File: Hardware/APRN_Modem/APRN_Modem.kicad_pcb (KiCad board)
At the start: 2 copper layers, 12 parts, among them J201 Conn_Coaxial, U201 VS1003, U202 DRA818V

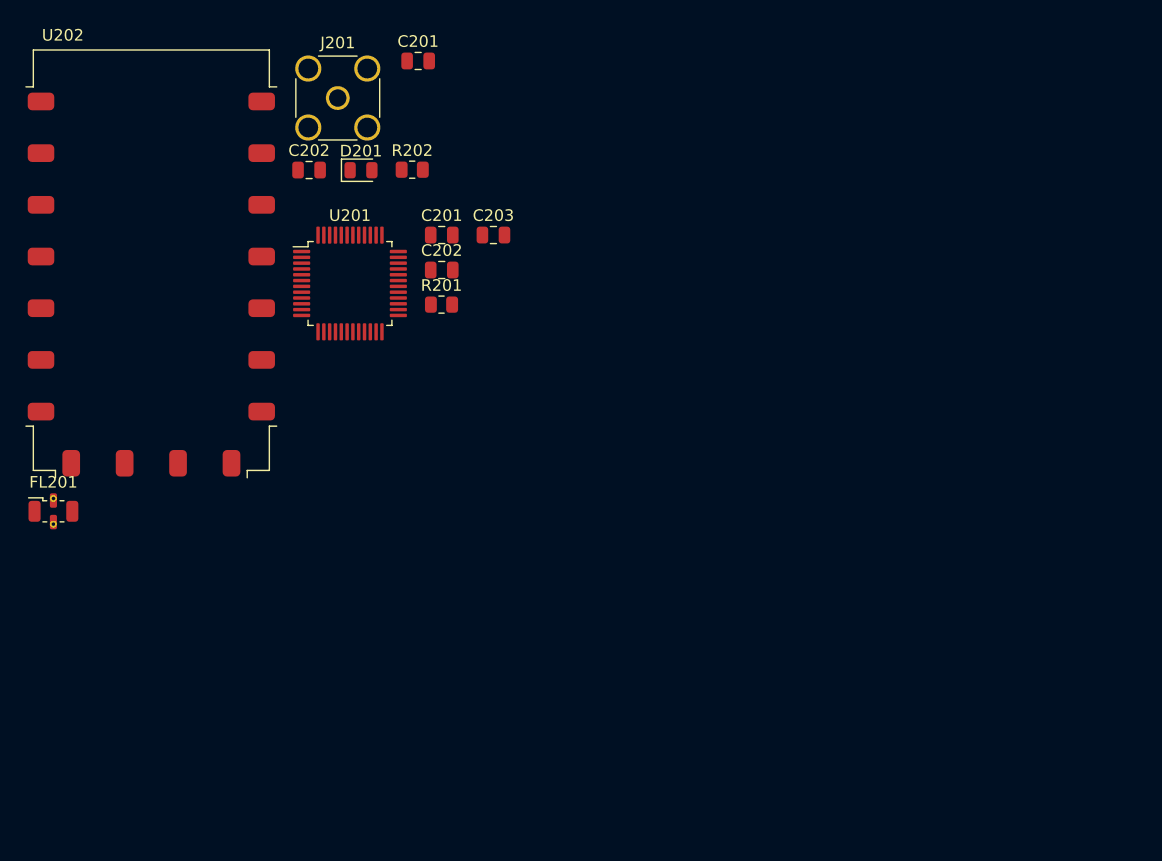
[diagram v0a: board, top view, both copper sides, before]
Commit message: Bump libs and stuff
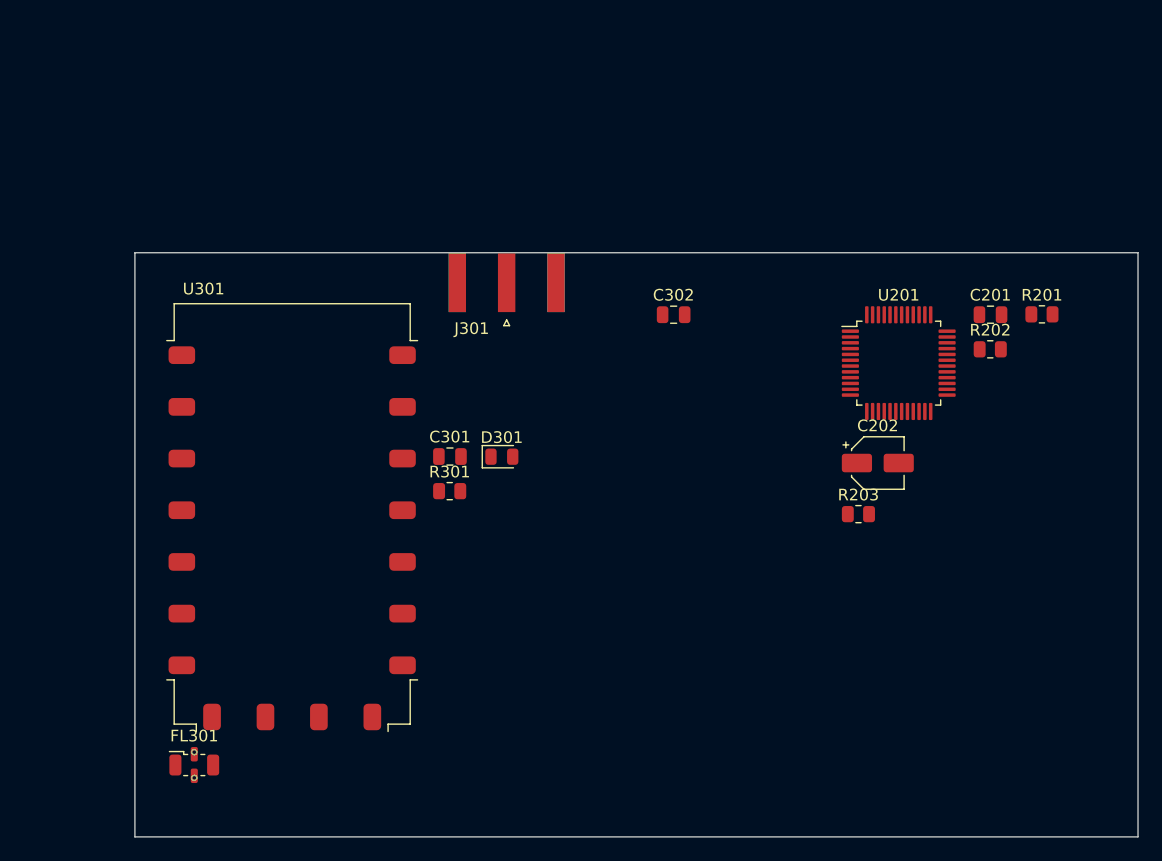
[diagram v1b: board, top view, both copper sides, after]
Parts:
- removed the C201 at (168.4, 81.3)
- removed the C201 at (170.4, 96.3)
- removed the C202 at (159.0, 90.7)
- removed the C202 at (170.4, 99.3)
- removed C203: 4.7uF, Capacitor_SMD:C_0805_2012Metric
- removed D201: RX, LED_SMD:LED_0805_2012Metric
- removed FL201: LFCN-490, Filter:Filter_Mini-Circuits_FV1206
- removed J201: Conn_Coaxial, Connector_Coaxial:SMA_Amphenol_132291_Vertical
- removed U202: DRA818V, KenwoodFox:DRA818V
- added C201: 1uF, Capacitor_SMD:C_0805_2012Metric, F.Cu at (217.7, 103.1)
- added C202: 10uf, Capacitor_SMD:CP_Elec_4x3, F.Cu at (208.0, 115.9)
- added C301: 100pF, Capacitor_SMD:C_0805_2012Metric, F.Cu at (171.1, 115.3)
- added C302: 4.7uF, Capacitor_SMD:C_0805_2012Metric, F.Cu at (190.4, 103.1)
- added D301: RX, LED_SMD:LED_0805_2012Metric, F.Cu at (175.6, 115.3)
- added FL301: LFCN-490, Filter:Filter_Mini-Circuits_FV1206, F.Cu at (149.1, 141.9)
- added J301: Conn_Coaxial, Connector_Coaxial:SMA_Amphenol_132289_EdgeMount, F.Cu at (176.0, 100.4)
- added R203: 100K, Resistor_SMD:R_0805_2012Metric, F.Cu at (206.3, 120.3)
- added R301: 2K2, Resistor_SMD:R_0805_2012Metric, F.Cu at (171.1, 118.3)
- added U301: DRA818V, KenwoodFox:DRA818V, F.Cu at (157.6, 120.0)
- R202: value 2K2 -> 100K
- moved R202 52.1 mm to (217.7, 106.1)
- moved R201 51.7 mm to (222.1, 103.1)
- moved U201 47.7 mm to (209.8, 107.3)
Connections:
- R201 pad 1: Net-(R201-Pad1) -> /VS1003/~{xRESET}
- R202 pad 1: +3.3V -> Net-(R202-Pad1)
- R202 pad 2: Net-(D201-Pad2) -> GND
- U201 pad 13: unconnected-(U201-Pad13) -> /VS1003/~{xDCS}
- U201 pad 14: unconnected-(U201-Pad14) -> /VS1003/IOVDD
- U201 pad 19: unconnected-(U201-Pad19) -> /VS1003/IOVDD
- U201 pad 23: unconnected-(U201-Pad23) -> /VS1003/~{xCS}
- U201 pad 24: unconnected-(U201-Pad24) -> /VS1003/CVDD
- U201 pad 26: unconnected-(U201-Pad26) -> Net-(R203-Pad2)
- U201 pad 28: unconnected-(U201-Pad28) -> /VS1003/SCLK
- U201 pad 29: unconnected-(U201-Pad29) -> /VS1003/SI
- U201 pad 3: unconnected-(U201-Pad3) -> /VS1003/~{xRESET}
- U201 pad 30: unconnected-(U201-Pad30) -> /VS1003/SO
- U201 pad 31: unconnected-(U201-Pad31) -> /VS1003/CVDD
- U201 pad 32: unconnected-(U201-Pad32) -> /VS1003/IOVDD
- U201 pad 33: Net-(R201-Pad1) -> Net-(R202-Pad1)
- U201 pad 38: unconnected-(U201-Pad38) -> /VS1003/AVDD
- U201 pad 43: unconnected-(U201-Pad43) -> /VS1003/AVDD
- U201 pad 45: unconnected-(U201-Pad45) -> /VS1003/AVDD
- U201 pad 5: unconnected-(U201-Pad5) -> /VS1003/CVDD
- U201 pad 6: unconnected-(U201-Pad6) -> /VS1003/IOVDD
- U201 pad 7: unconnected-(U201-Pad7) -> /VS1003/CVDD
- U201 pad 8: unconnected-(U201-Pad8) -> /VS1003/DREQ
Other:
- board outline added: 86.4 x 50.3 mm
